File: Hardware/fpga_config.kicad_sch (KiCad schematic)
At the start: 1 part, among them U2 XC7A35T-CSG325

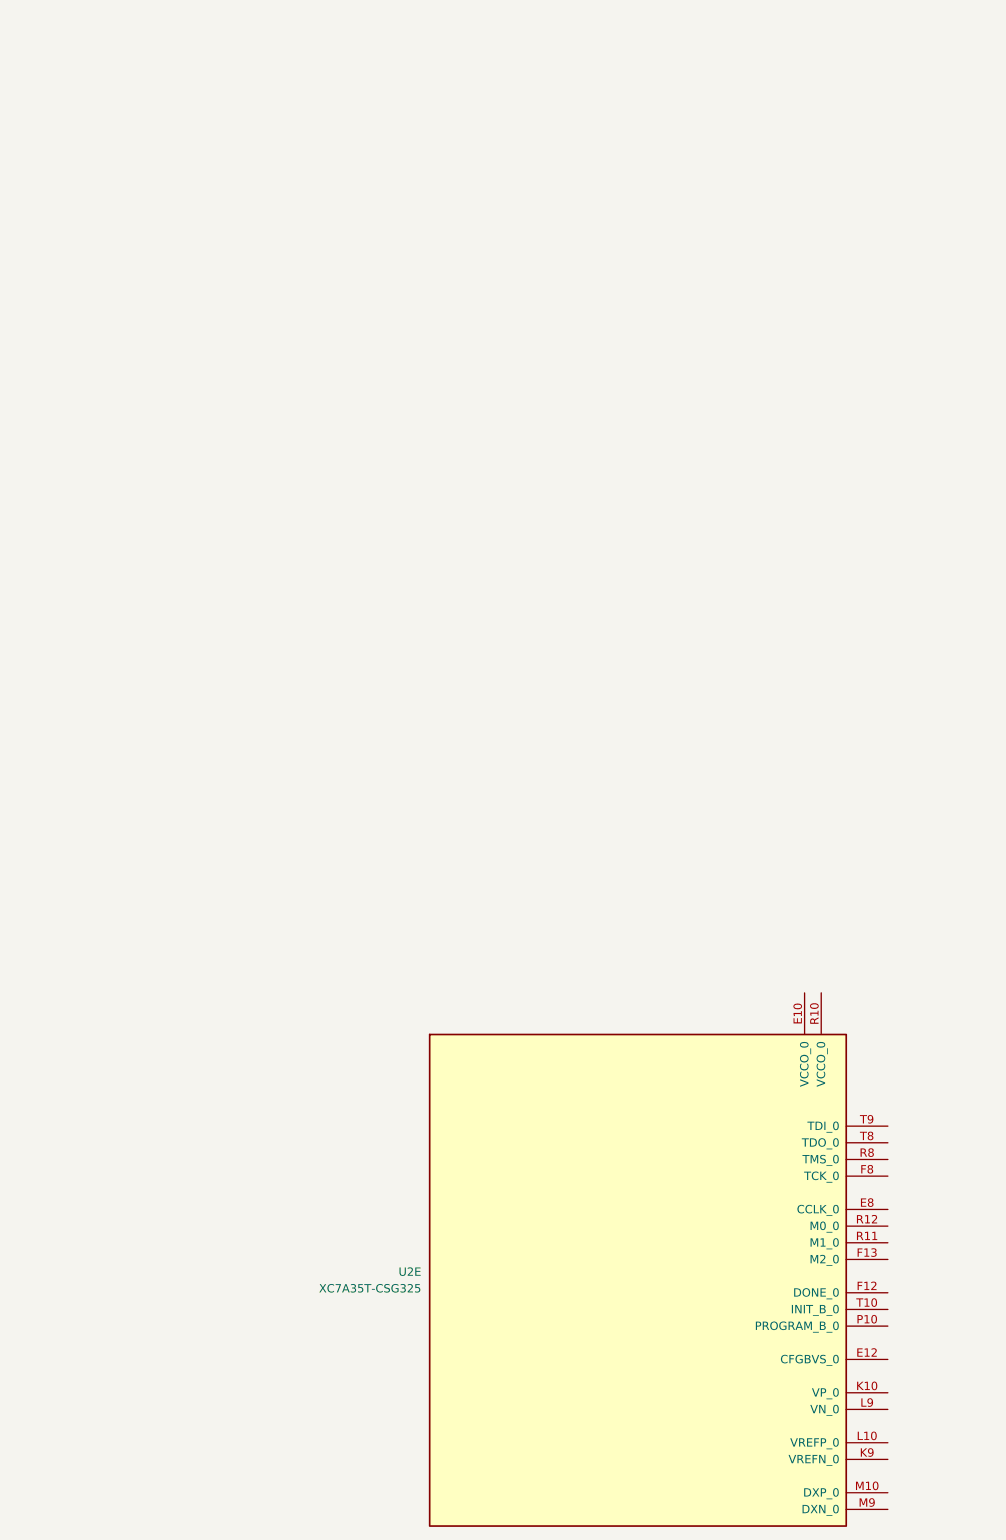
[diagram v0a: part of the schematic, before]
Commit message: PCIe
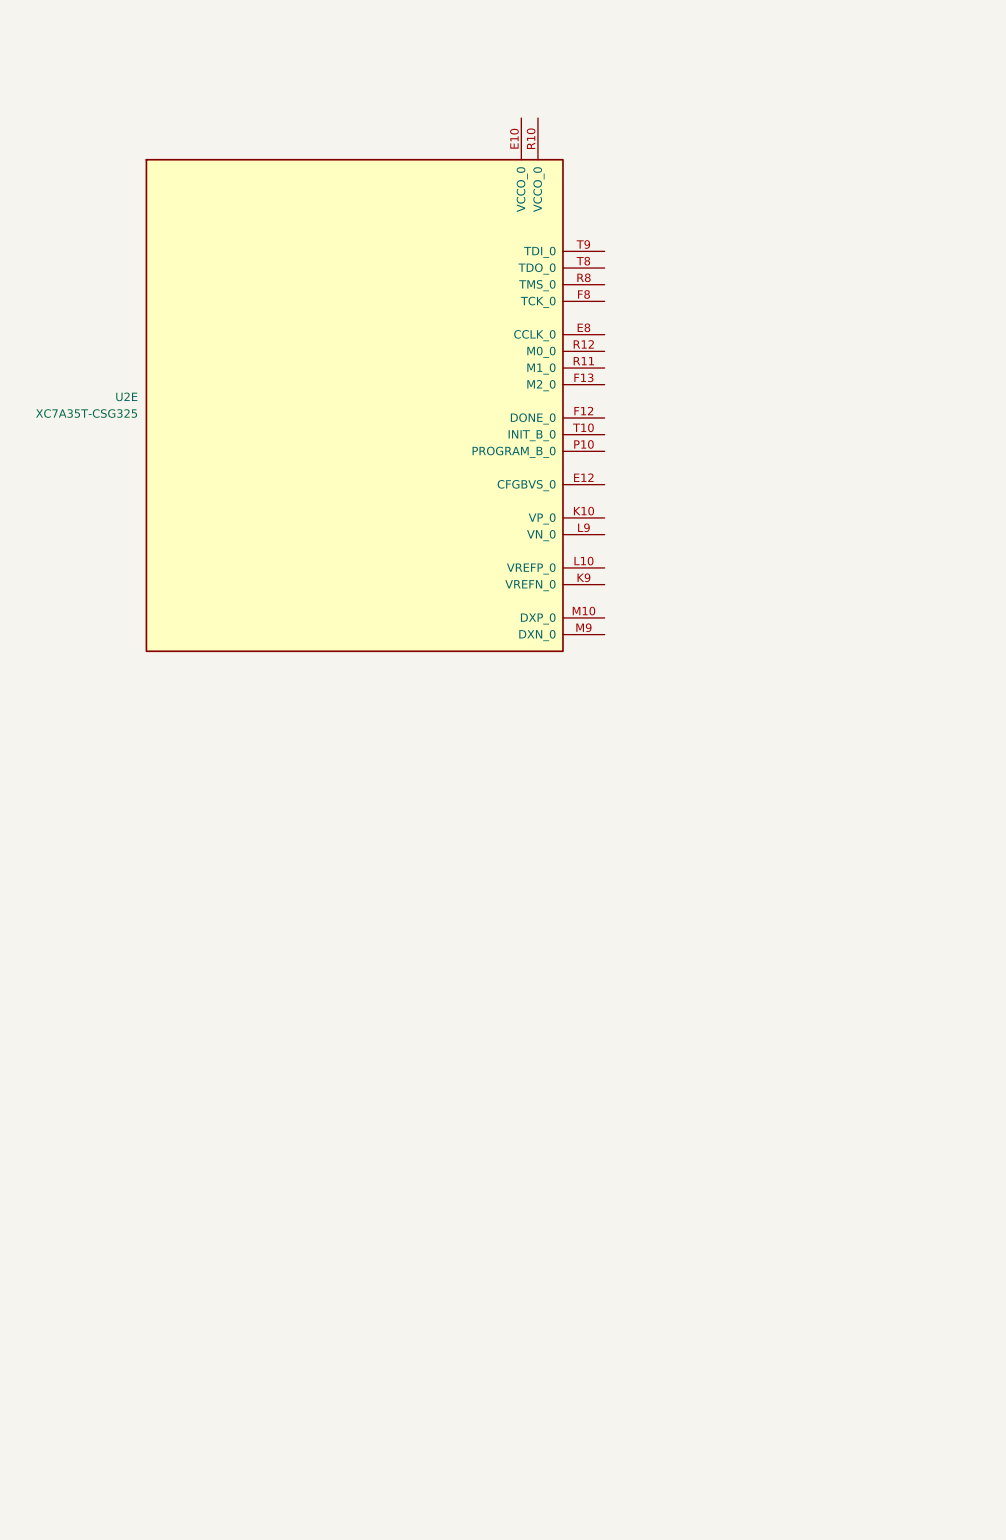
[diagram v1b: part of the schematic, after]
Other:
- moved on the sheet: U2E
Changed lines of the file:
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@@
 	(symbol
 		(lib_id "FPGA_Xilinx_Artix7:XC7A35T-CSG325")
-		(at 167.64 223.52 0)
+		(at 124.46 90.17 0)
 		(unit 5)
 		(body_style 1)
@@
 		(fields_autoplaced yes)
 		(property "Reference" "U2"
-			(at 134.62 225.4249 0)
+			(at 91.44 92.0749 0)
 			(show_name no)
 			(do_not_autoplace no)
@@
 		)
 		(property "Value" "XC7A35T-CSG325"
-			(at 134.62 227.9649 0)
+			(at 91.44 94.6149 0)
 			(show_name no)
 			(do_not_autoplace no)
@@
 		)
 		(property "Footprint" "Package_BGA:Xilinx_CSG325"
-			(at 167.64 223.52 0)
+			(at 124.46 90.17 0)
 			(hide yes)
 			(show_name no)
@@
 		)
 		(property "Datasheet" ""
-			(at 167.64 223.52 0)
+			(at 124.46 90.17 0)
 			(show_name no)
 			(do_not_autoplace no)
@@
 		)
 		(property "Description" "Artix 7 T 35 XC7A35T-CSG325"
-			(at 167.64 223.52 0)
+			(at 124.46 90.17 0)
 			(hide yes)
 			(show_name no)
